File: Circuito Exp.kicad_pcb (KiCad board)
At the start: 2 copper layers, 83.8 x 50.8 mm, 13 parts, among them M1 Microfone, P1 DIL8, SW1 SPST

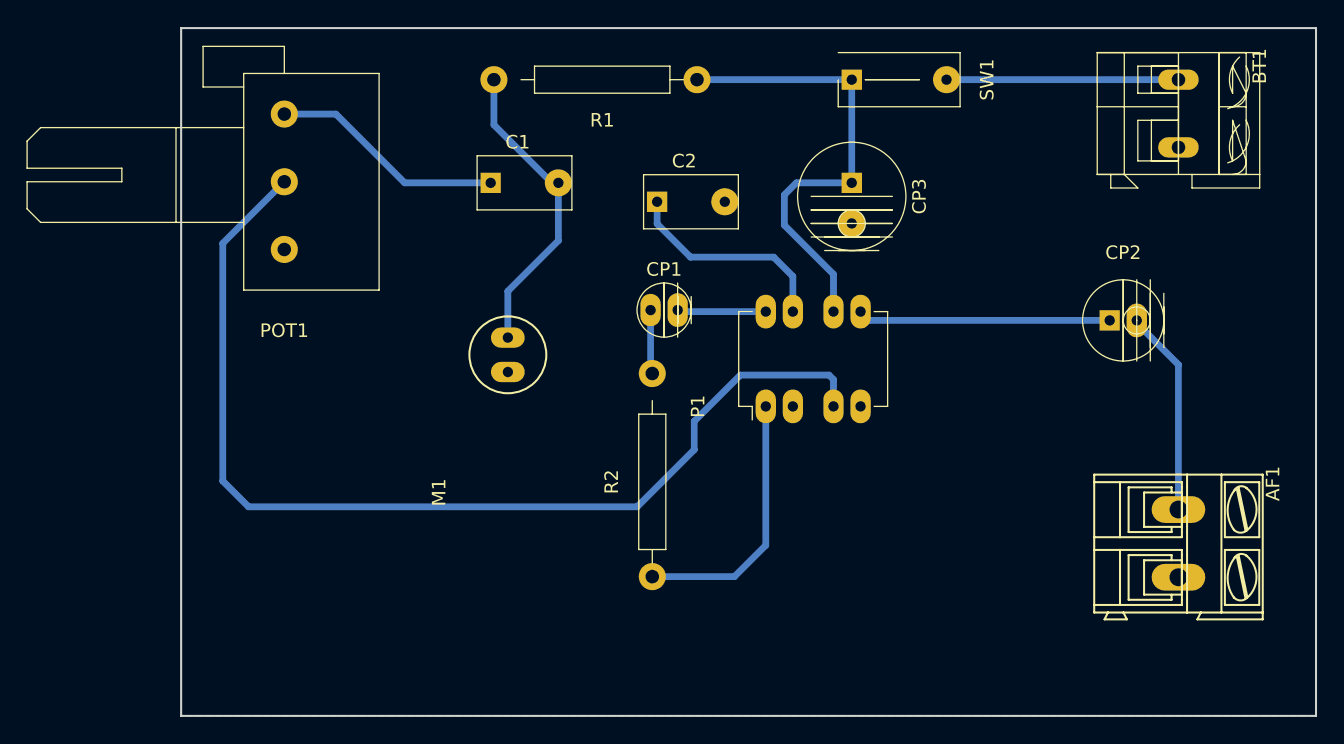
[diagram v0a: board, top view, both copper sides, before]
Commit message: 100%
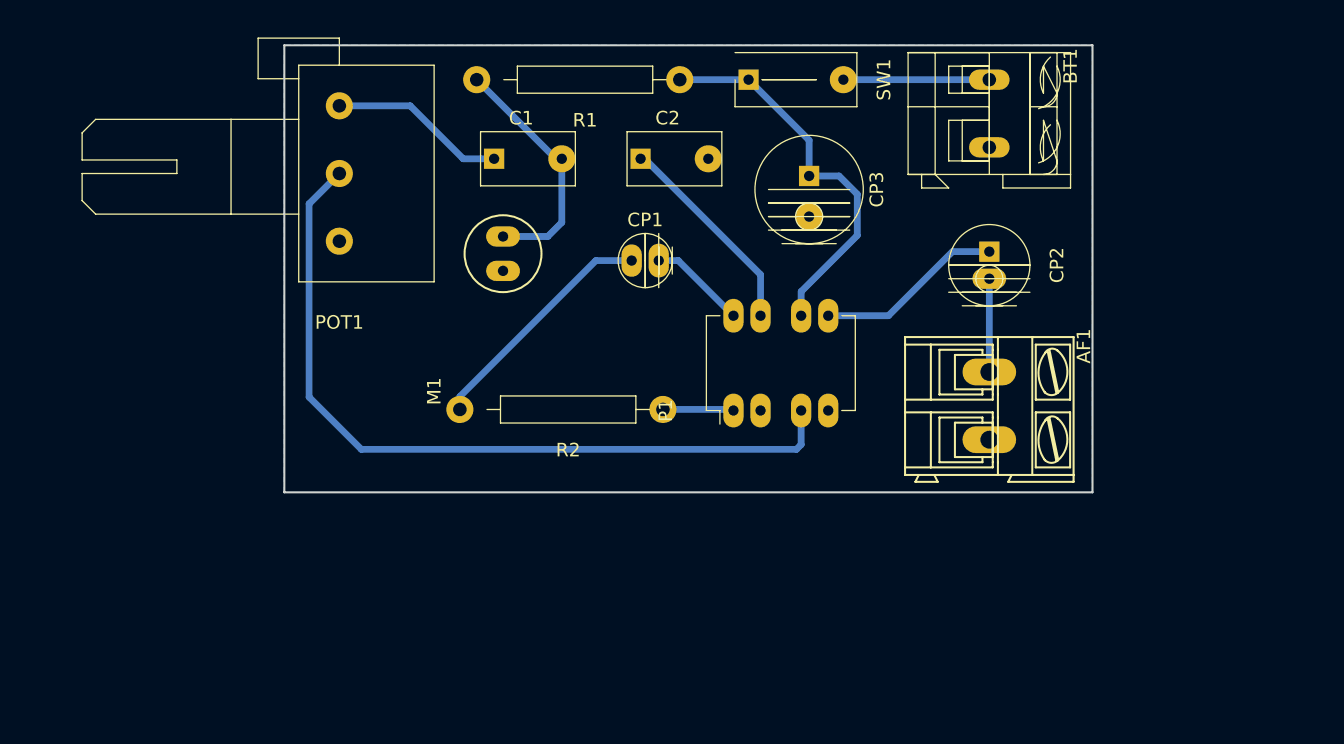
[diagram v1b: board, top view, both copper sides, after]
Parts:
- moved AF1 17.3 mm to (176.5, 88.9)
- moved BT1 14.0 mm to (176.5, 67.3)
- moved R2 12.4 mm to (152.4, 91.7), turned to 180 degrees
- moved CP2 10.2 mm to (176.5, 80.0), turned to 270 degrees
- moved SW1 7.62 mm to (158.8, 67.3)
- moved M1 7.48 mm to (140.6, 81.4)
- moved POT1 4.11 mm to (128.5, 69.2)
- moved CP1 3.92 mm to (150.1, 80.7)
- moved C2 3.40 mm to (150.8, 73.2)
- moved CP3 3.19 mm to (163.2, 74.4)
- moved P1 2.41 mm to (157.6, 91.7)
- moved C1 1.80 mm to (140.0, 73.2)
- moved R1 1.27 mm to (153.7, 67.3)
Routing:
- net Net-(P1-Pad3): track 77.3 -> 58.0 mm
- net Net-(P1-Pad1): track 19.6 -> 5.24 mm
- net Net-(CP1-Pad1): track 4.74 -> 17.8 mm
- net Net-(AF1-Pad1): track 15.2 -> 6.89 mm
- net /VCC: track 35.5 -> 28.9 mm
- net Net-(BT1-Pad1): track 17.1 -> 10.8 mm
- net Net-(CP2-Pad1): track 18.7 -> 13.9 mm
- net Net-(C1-Pad2): track 22.8 -> 18.2 mm
- net Net-(C1-Pad1): track 17.3 -> 13.1 mm
- net Net-(CP1-Pad2): track 6.56 -> 7.21 mm
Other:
- board size 83.8 x 50.8 mm -> 59.7 x 33 mm
